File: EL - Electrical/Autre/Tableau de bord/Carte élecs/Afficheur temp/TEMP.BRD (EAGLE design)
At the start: 79 x 42 mm, 25 parts, among them IC1 MCP23008P, IC2 MCP23008P, X1 22-23-2041

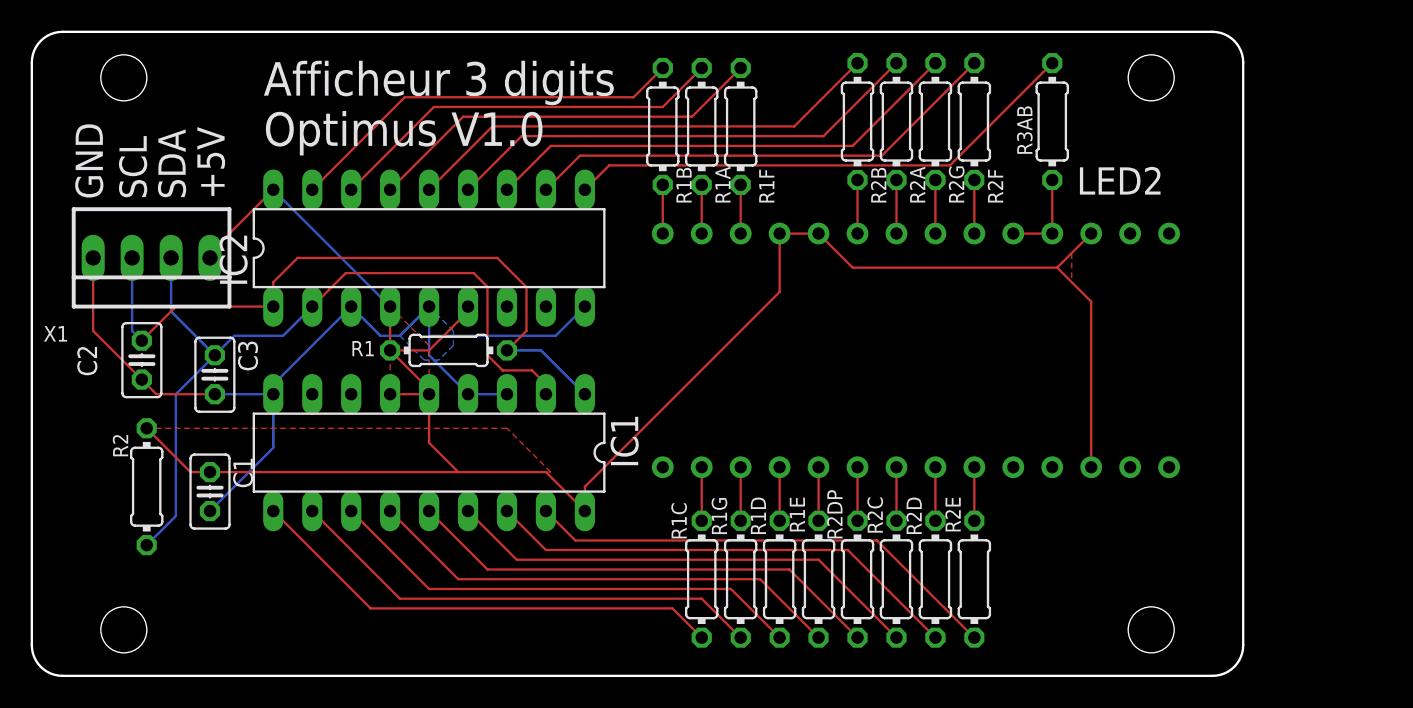
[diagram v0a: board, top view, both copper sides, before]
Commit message: MAJ plan afficheur temp
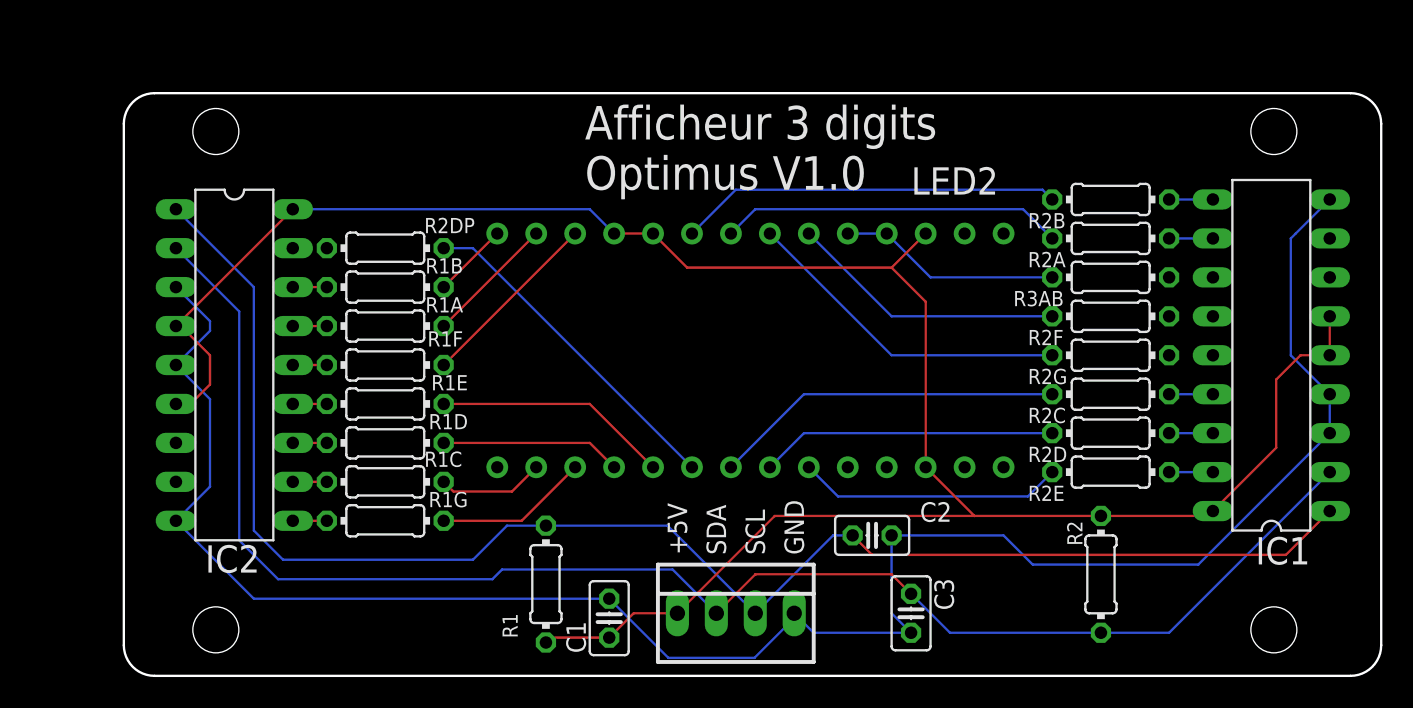
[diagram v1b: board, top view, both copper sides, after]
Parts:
- moved R2 62.5 mm to (65.7, 7.62)
- moved IC1 55.3 mm to (76.8, 21.9), turned to 90 degrees
- moved C2 49.0 mm to (50.8, 10.2), turned to 0 degrees
- moved C3 48.0 mm to (53.3, 5.08)
- moved X1 44.6 mm to (41.9, 5.08), turned to 0 degrees
- moved R2DP 37.6 mm to (19.1, 28.9), turned to 0 degrees
- moved R1E 30.5 mm to (19.1, 18.7), turned to 180 degrees
- moved R1F 27.9 mm to (19.1, 21.3), turned to 180 degrees
- moved C1 27.3 mm to (33.7, 4.76), turned to 90 degrees
- moved R1D 27.2 mm to (19.1, 16.2), turned to 180 degrees
- moved R1A 24.4 mm to (19.1, 23.8), turned to 180 degrees
- moved R1G 23.5 mm to (19.1, 11.1), turned to 180 degrees
- moved R1C 21.6 mm to (19.1, 13.7), turned to 180 degrees
- moved R1B 20.9 mm to (19.1, 26.4), turned to 180 degrees
- moved R2G 19.1 mm to (66.4, 21.9), turned to 0 degrees
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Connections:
- net GP10: now also R2B.2; no longer R1C.2
- net GP11: now also R2A.2; no longer R1G.2
- net GP12: now also R3AB.2; no longer R1D.2
- net GP13: now also R2F.2; no longer R1E.2
- net GP14: now also R2G.2; no longer R2DP.1
- net GP20: now also R1G.2; no longer R3AB.2
- net GP21: now also R1C.2; no longer R2F.2
- net GP22: now also R1D.2; no longer R2G.2
- net GP23: now also R1E.2; no longer R2A.2
- net GP24: now also R1F.2; no longer R2B.2
- net GP25: now also R1A.2; no longer R1F.2
- net GP26: now also R1B.2; no longer R1A.2
- net GP27: now also R2DP.1; no longer R1B.2
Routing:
- net GND: track 63.2 -> 129.5 mm
- net SCL: track 45.6 -> 101.1 mm
- net SDA: track 52.5 -> 101.3 mm
- net GP20: track 33.9 -> 2.22 mm
- net GP12: track 31.4 -> 0.00 mm
- net GP14: track 31.4 -> 0.00 mm
- net GP13: track 31.4 -> 0.00 mm
- net GP23: track 31.4 -> 2.22 mm
- net GP22: track 31.4 -> 2.22 mm
- net GP21: track 31.4 -> 2.22 mm
- net GP24: track 31.4 -> 2.22 mm
- net GP17: track 31.4 -> 2.86 mm
- net GP16: track 31.4 -> 2.86 mm
- net GP15: track 31.4 -> 2.86 mm
- net GP11: track 31.4 -> 2.86 mm
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- removed copper zone on layer 1, net +5V
- removed copper zone on layer 16, net GND
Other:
- board size 79 x 42 mm -> 82 x 38 mm
